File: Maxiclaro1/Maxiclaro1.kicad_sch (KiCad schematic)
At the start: 33 parts, among them K1 SRD-05VDC-SL-C, K2 SRD-05VDC-SL-C, K3 SRD-05VDC-SL-C, K4 SRD-05VDC-SL-C, Q1 BC547, Q2 BC547, Q3 BC547, Q4 BC547, U1 ESP32-DEVKITC-32D

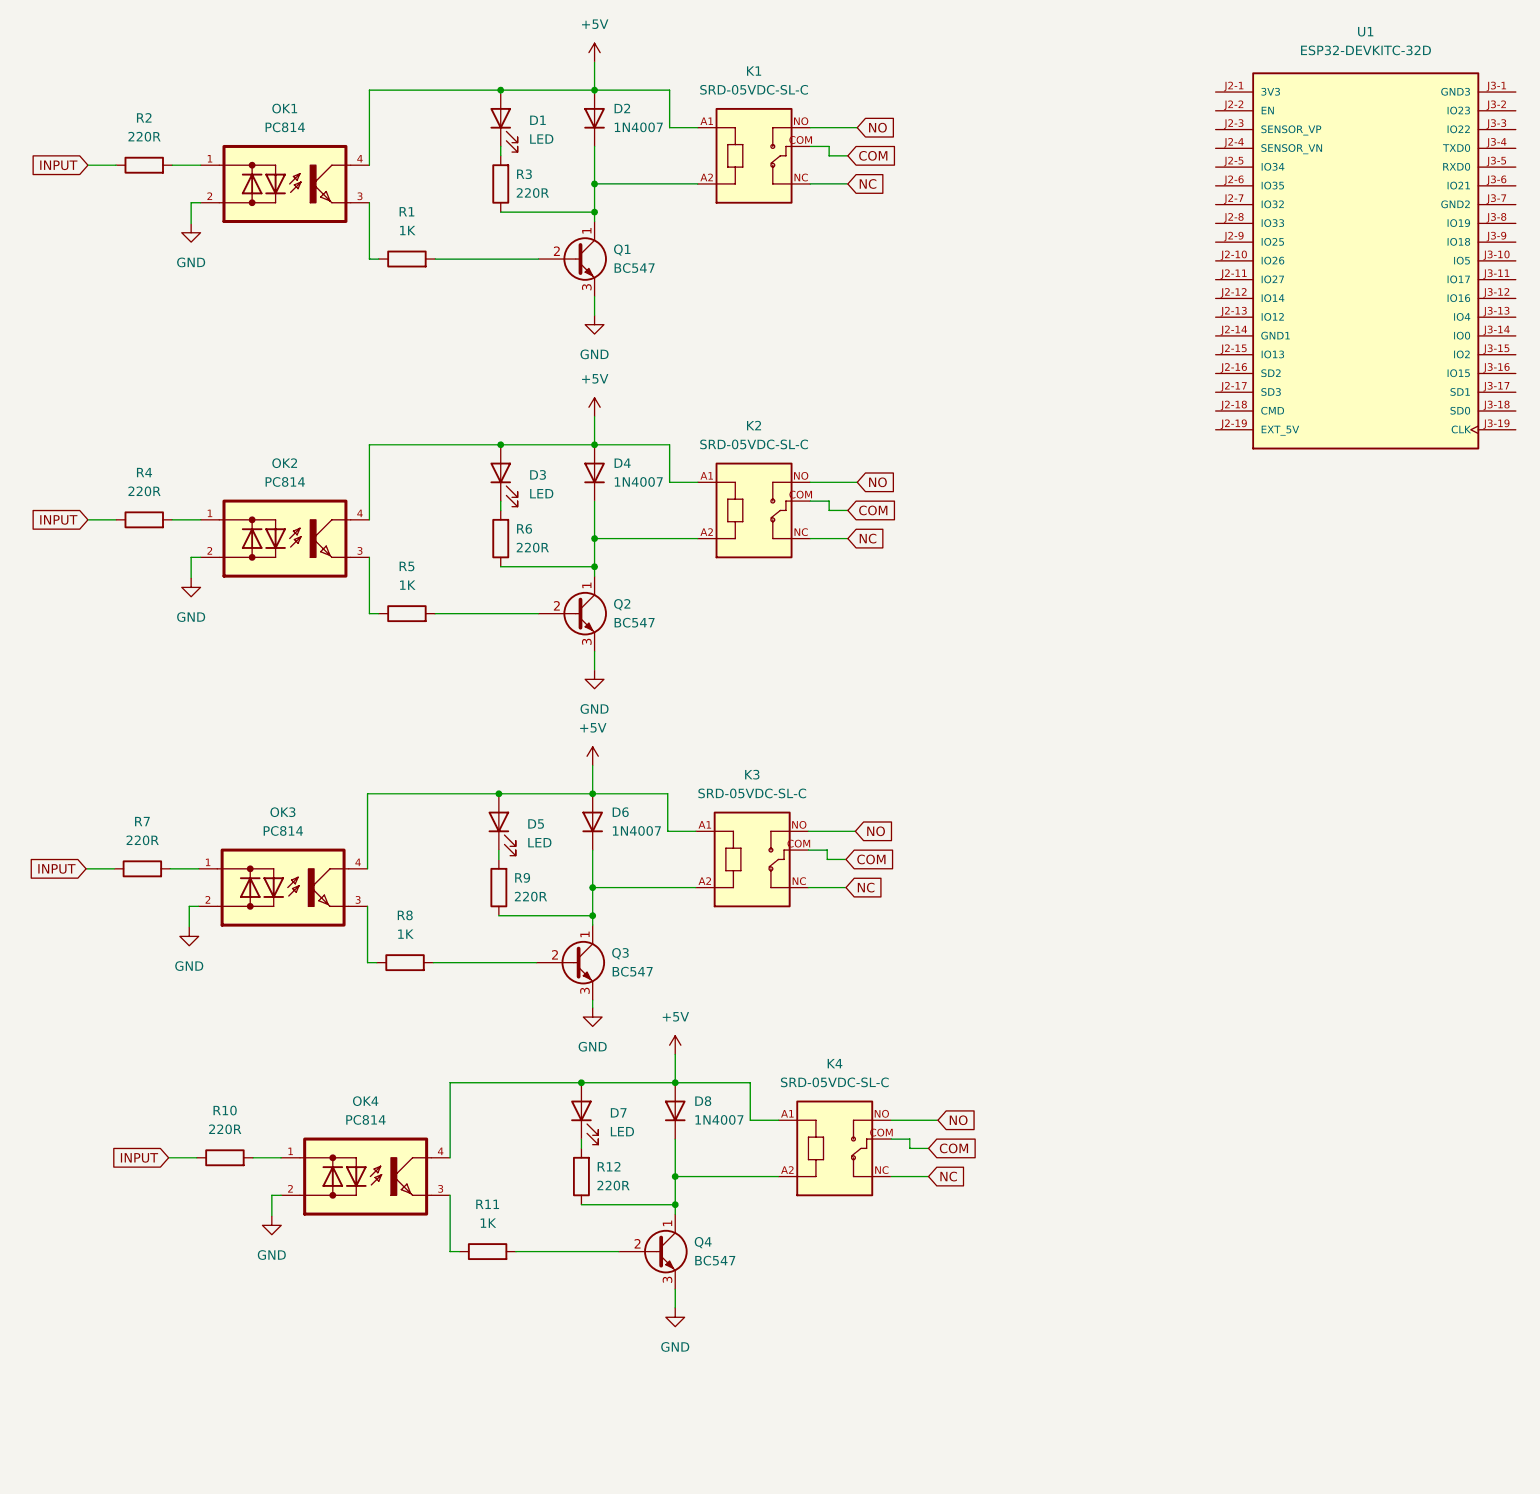
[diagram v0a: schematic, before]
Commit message: Add files via upload
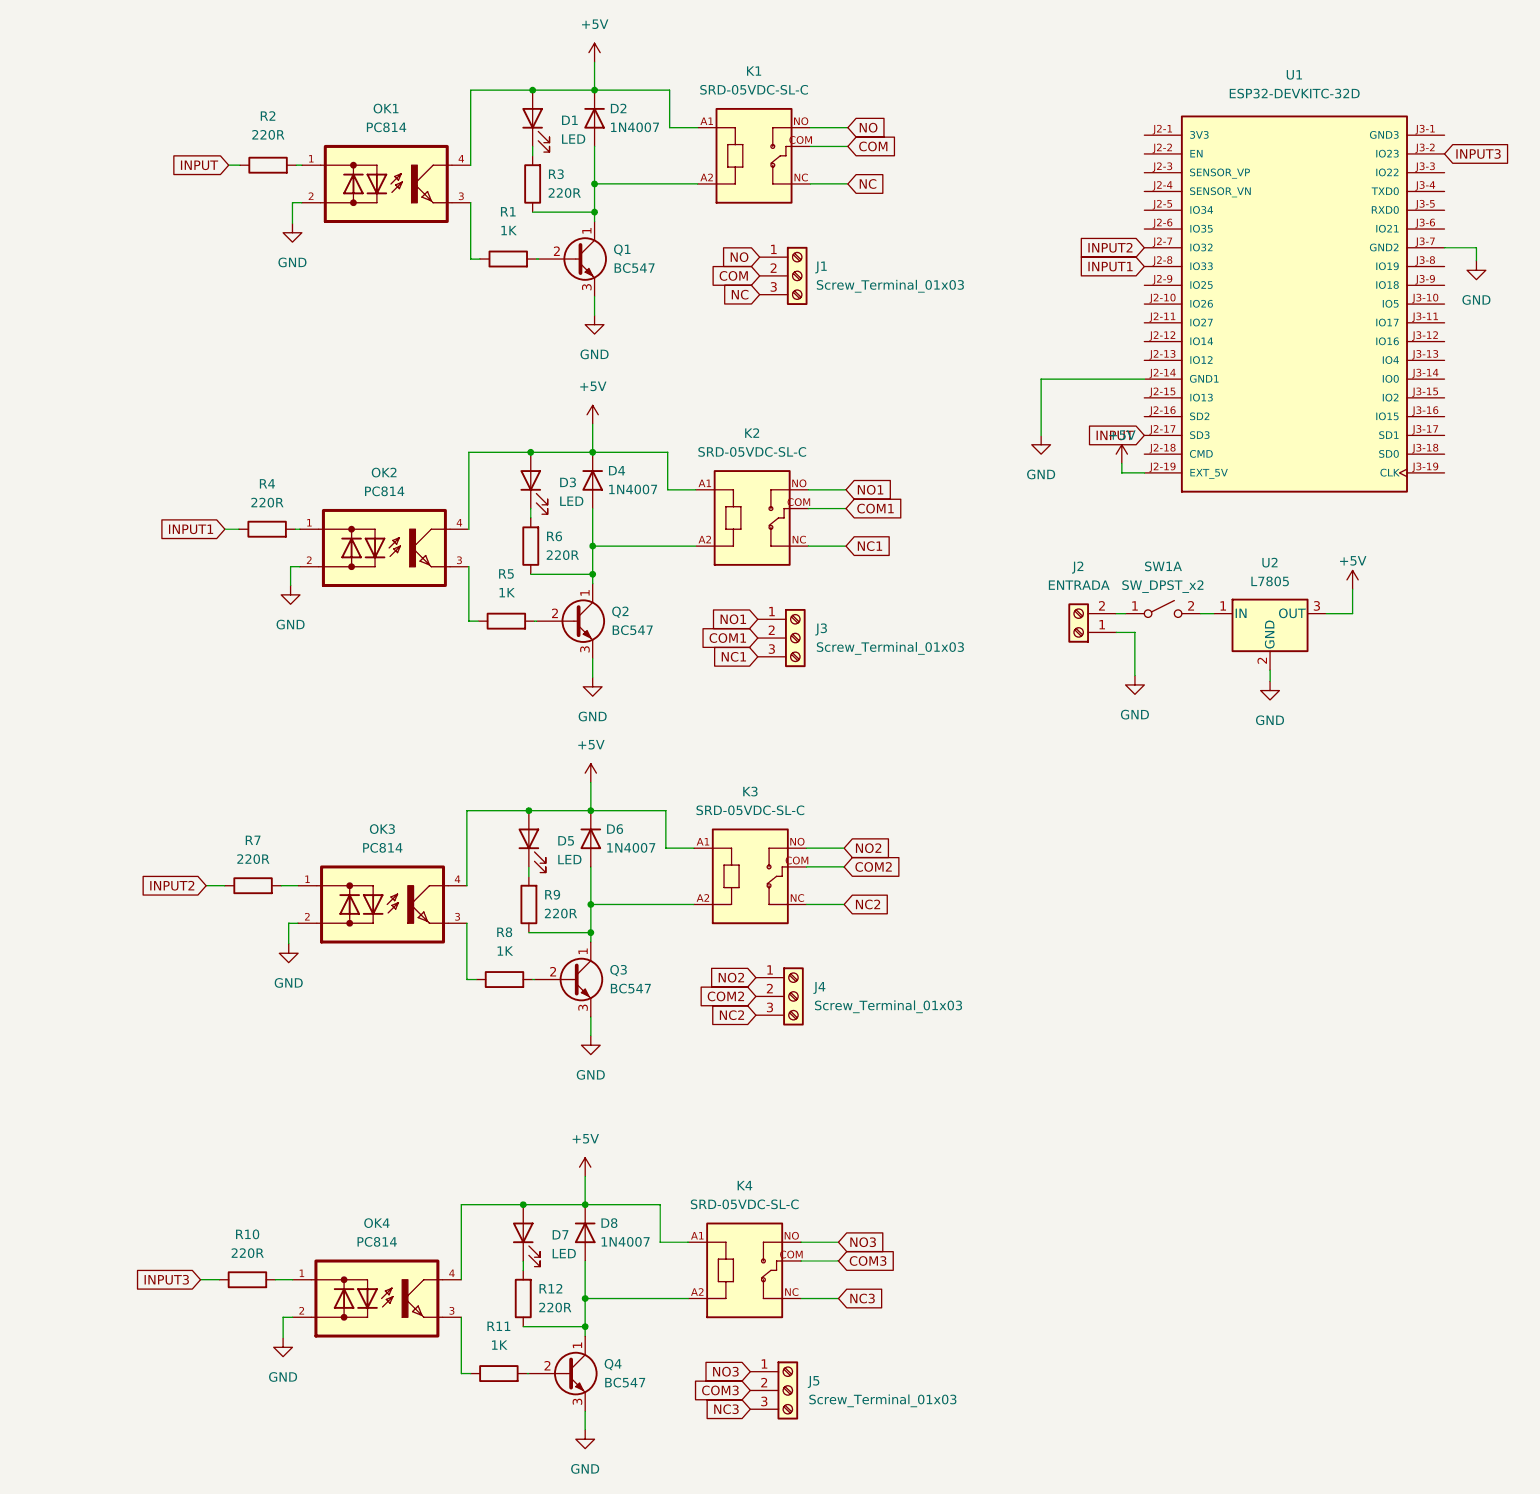
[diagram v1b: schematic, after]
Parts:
- added J1, J3, J4, J5: Screw_Terminal_01x03, TerminalBlock:TerminalBlock_bornier-3_P5.08mm, symbol Connector:Screw_Terminal_01x03
- added J2: ENTRADA, TerminalBlock:TerminalBlock_Altech_AK300-2_P5.00mm, symbol Connector:Screw_Terminal_01x02
- added SW1: SW_DPST_x2, 2MS1T1B1M2QES:SW_2MS1T1B1M2QES-5, symbol Switch:SW_DPST_x2
- added U2: L7805, Package_TO_SOT_SMD:TO-263-2, symbol Regulator_Linear:L7805
- D1, D3, D5, D7: footprint EESTN5:Led_0805 -> LED_SMD:LED_0805_2012Metric
- D2, D4, D6, D8: footprint OptoDevice:R_LDR_4.9x4.2mm_P2.54mm_Vertical -> Diode_SMD:D_0805_2012Metric
- K1, K2: footprint SRD-05VDC-SL:RELAY_SRD-05VDC-SL-C -> SRD-05VDC-SL-C:RELAY_SRD-05VDC-SL-C
- K3: footprint SRD-05VDC-SL:RELAY_SRD-05VDC-SL-C -> RELAY:RELAY_SRD-05VDC-SL-C
- K4: footprint SRD-05VDC-SL:RELAY_SRD-05VDC-SL-C -> RELAY_SRD-05VDC-SL-C:RELAY_SRD-05VDC-SL-C
- OK3, OK4: footprint PC814:DIL04 -> DIL04:DIL04
- R1, R10, R11, R12, R2, R3, R4, R5, R6, R7, R8, R9: footprint EESTN5:R_0805 -> Resistor_SMD:R_0805_2012Metric
- U1: footprint ESP32-DEVKITC-32D:MODULE_ESP32-DEVKITC-32D -> ESP32−DEVKITC32D:MODULE_ESP32-DEVKITC-32D
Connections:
- net +5V: now also D2.1 (K), D4.1 (K), D6.1 (K), D8.1 (K), U1.J2-19 (EXT_5V), U2.3 (OUT); no longer D2.2 (A), D4.2 (A), D6.2 (A), D8.2 (A)
- net COM: now also J1.2 (Pin_2); no longer K2.COM, K3.COM, K4.COM
- net GND: now also U1.J2-14 (GND1), U1.J3-7 (GND2), J2.1 (Pin_1), U2.2 (GND)
- net INPUT: now also U1.J2-17 (SD3); no longer R10.1, R4.1, R7.1
- net NC: now also J1.3 (Pin_3); no longer K2.NC, K3.NC, K4.NC
- net NO: now also J1.1 (Pin_1); no longer K2.NO, K3.NO, K4.NO
- net at K3.A2, Q3.1 (C), R9.1: now also D6.2 (A); no longer D6.1 (K)
- net at K2.A2, Q2.1 (C), R6.1: now also D4.2 (A); no longer D4.1 (K)
- net at K4.A2, Q4.1 (C), R12.1: now also D8.2 (A); no longer D8.1 (K)
- net INPUT2: now reaches U1.J2-7 (IO32)
- net INPUT2: now also R7.1
- net INPUT1: now reaches U1.J2-8 (IO33)
- net INPUT1: now also R4.1
- net INPUT3: now reaches U1.J3-2 (IO23)
- net INPUT3: now also R10.1
- net at K1.A2, Q1.1 (C), R3.1: now also D2.2 (A); no longer D2.1 (K)
- new net: J2.2 (Pin_2), SW1.1 (A)
- new net: SW1.2 (B), U2.1 (IN)
- new net COM1: J3.2 (Pin_2), K2.COM
- new net COM2: J4.2 (Pin_2), K3.COM
- new net COM3: J5.2 (Pin_2), K4.COM
- new net NC1: J3.3 (Pin_3), K2.NC
- new net NC2: J4.3 (Pin_3), K3.NC
- new net NC3: J5.3 (Pin_3), K4.NC
- new net NO1: J3.1 (Pin_1), K2.NO
- new net NO2: J4.1 (Pin_1), K3.NO
- new net NO3: J5.1 (Pin_1), K4.NO
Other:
- moved on the sheet: D1, D2, OK1, R1, R2, R3, U1
